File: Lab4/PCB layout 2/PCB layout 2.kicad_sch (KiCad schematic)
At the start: 10 parts, among them J1 Conn_01x02_Male, U1 NE555D

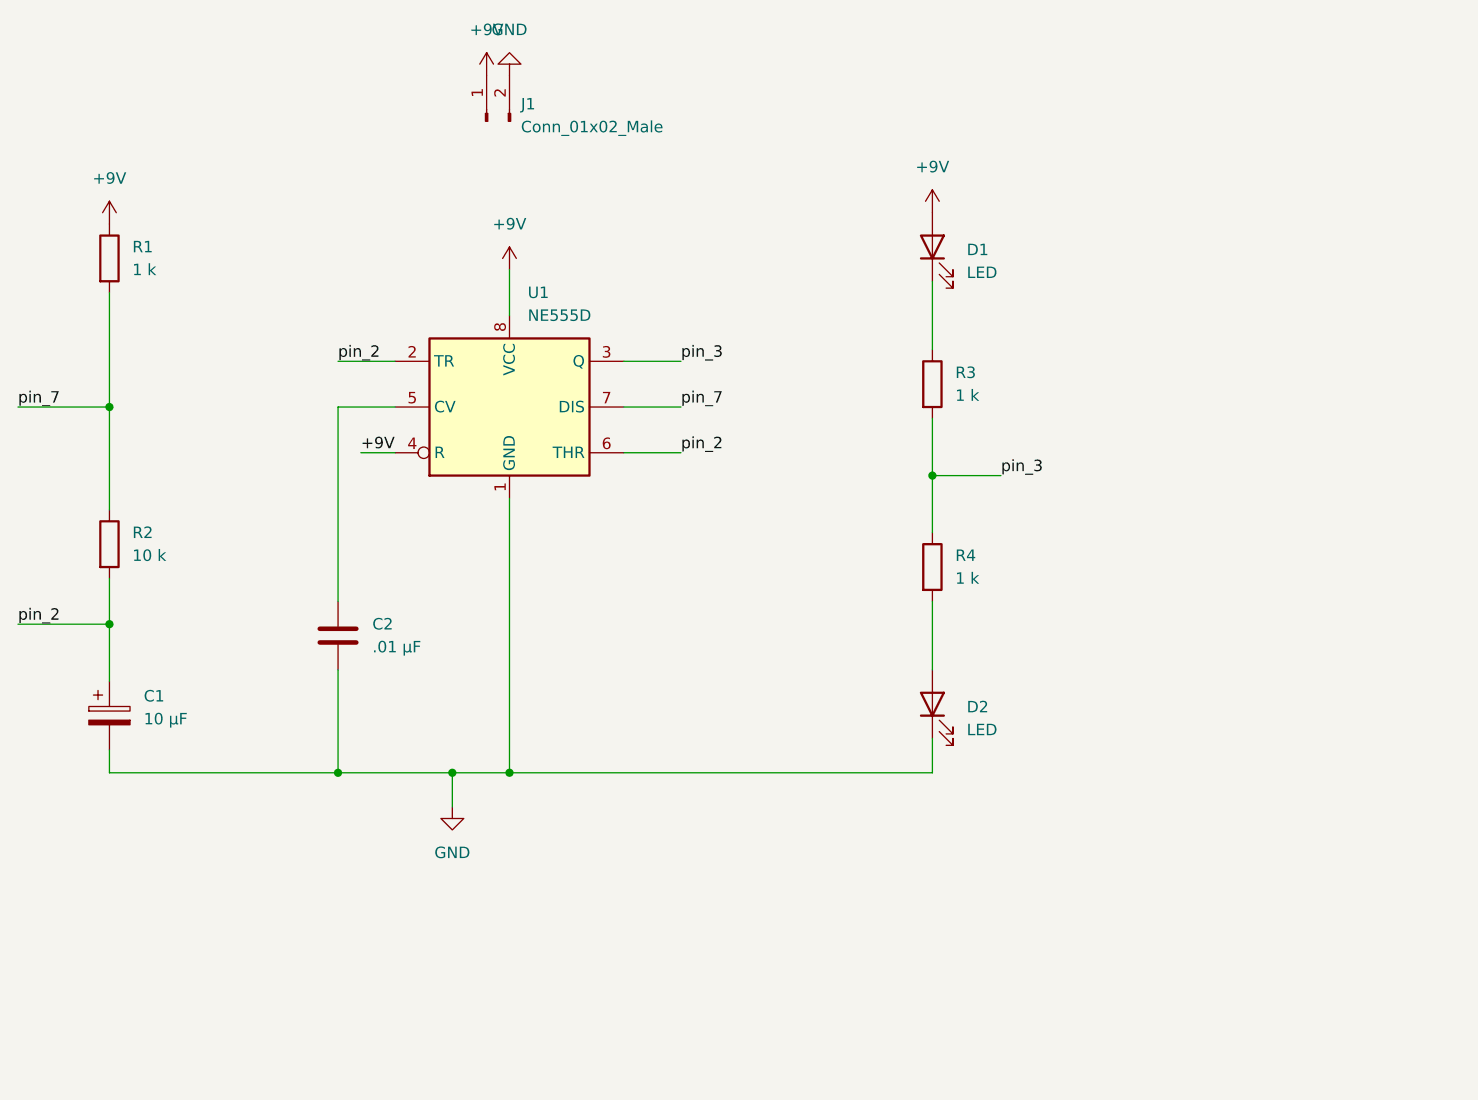
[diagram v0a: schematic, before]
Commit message: save both pcb layout
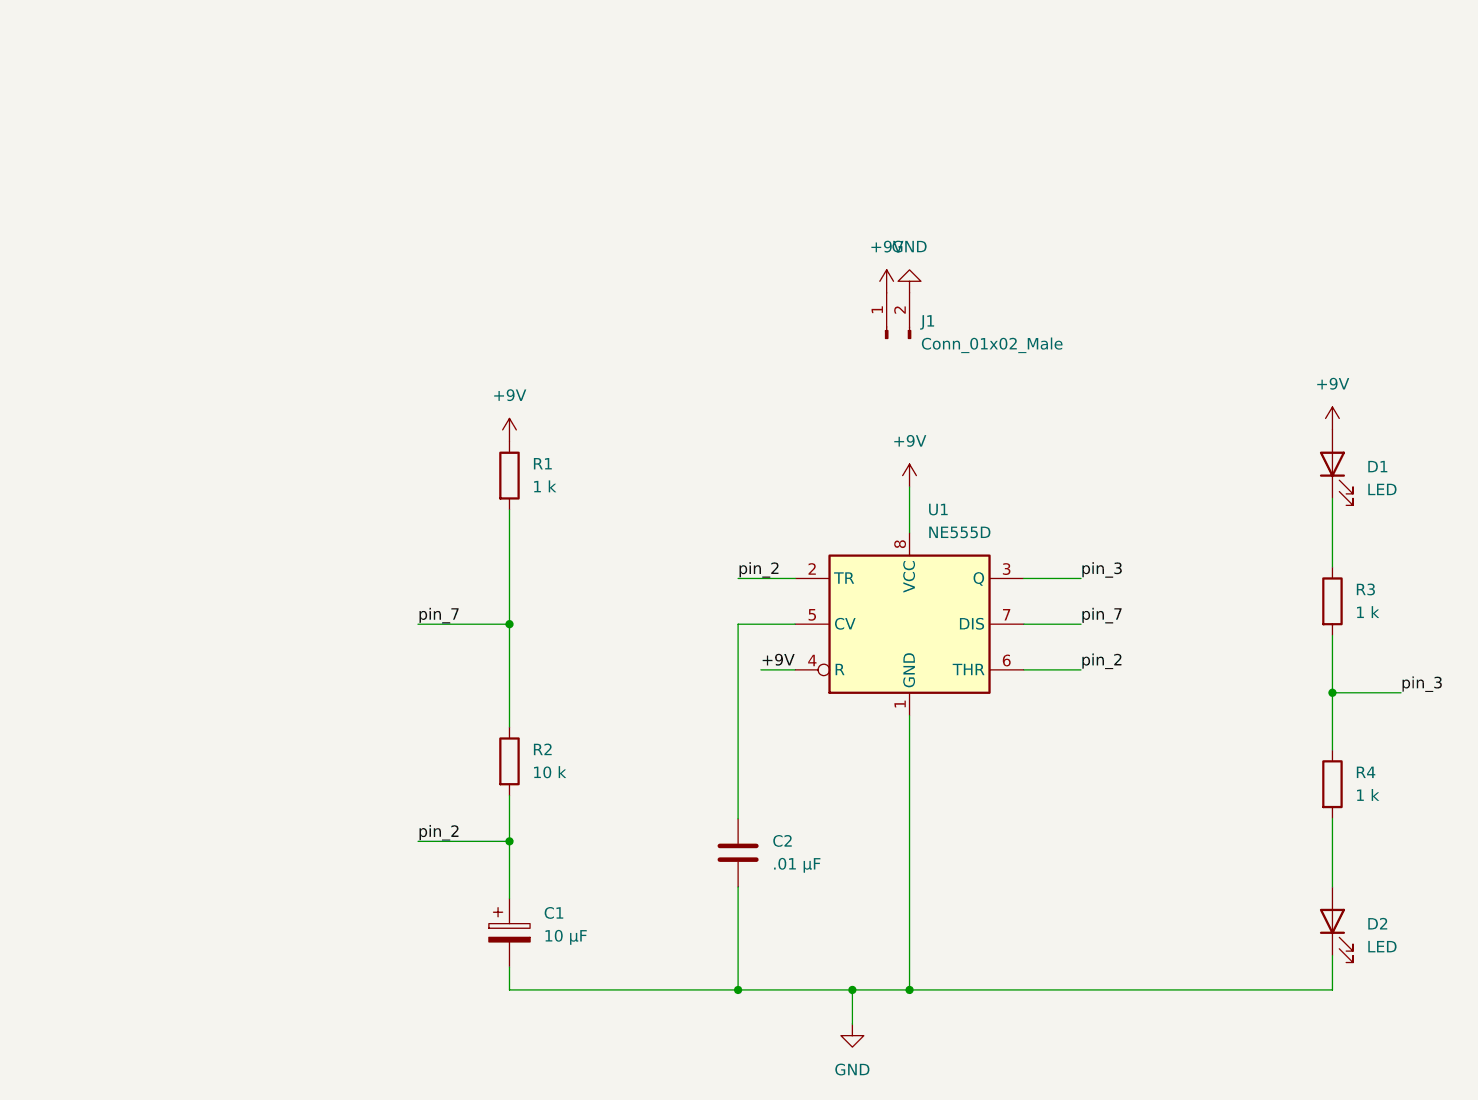
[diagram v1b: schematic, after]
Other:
- title: 555 Timer Circuit -> (none)
